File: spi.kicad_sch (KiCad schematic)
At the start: 15 parts, among them J3 Micro_SD_Card

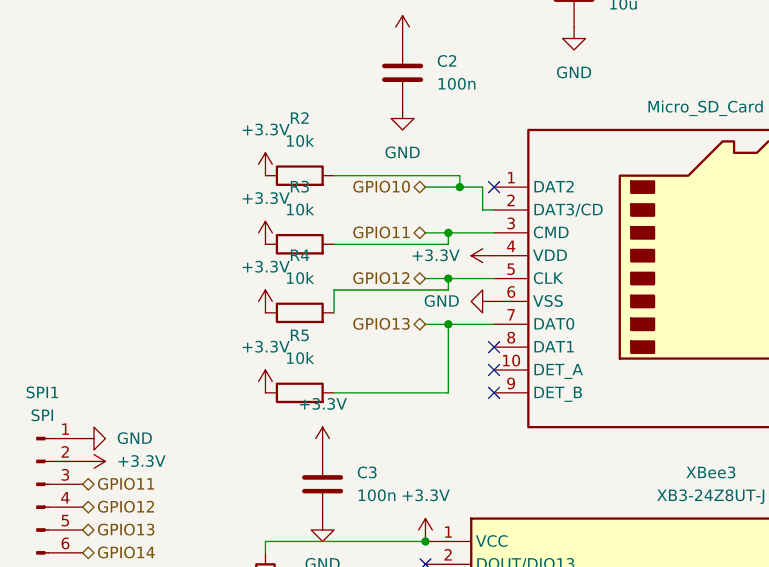
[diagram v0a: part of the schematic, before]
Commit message: Updated to v1.2 to address remaining issues
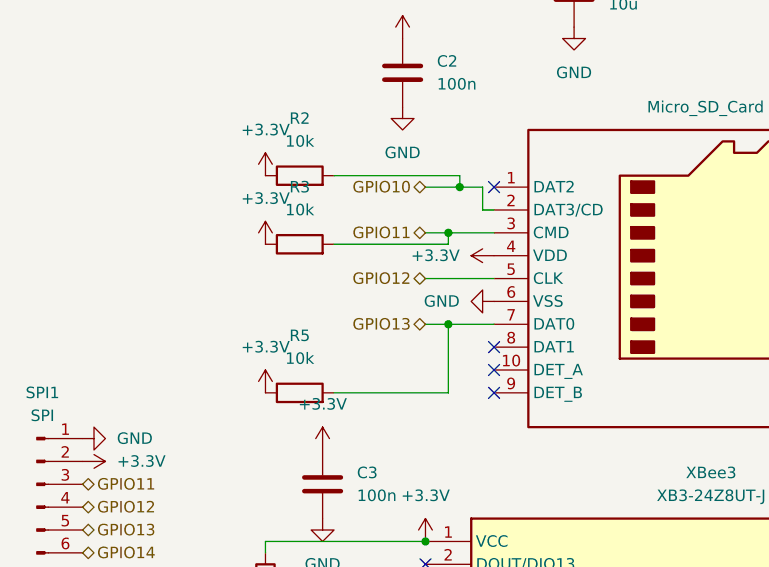
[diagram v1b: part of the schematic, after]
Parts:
- removed R4: 10k, Resistor_SMD:R_0603_1608Metric, symbol Device:R
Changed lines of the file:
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@@
 	)
 	(junction
-		(at 113.03 68.58)
-		(diameter 0)
-		(color 0 0 0 0)
-	)
-	(junction
 		(at 110.49 97.79)
 		(diameter 0)
@@
 	(wire
 		(pts
-			(xy 100.33 69.85) (xy 113.03 69.85)
-		)
-		(stroke
-			(width 0)
-			(type default)
-		)
-	)
-	(wire
-		(pts
 			(xy 113.03 81.28) (xy 113.03 73.66)
 		)
@@
 	(wire
 		(pts
-			(xy 100.33 72.39) (xy 100.33 69.85)
-		)
-		(stroke
-			(width 0)
-			(type default)
-		)
-	)
-	(wire
-		(pts
 			(xy 100.33 64.77) (xy 113.03 64.77)
 		)
@@
 	(wire
 		(pts
-			(xy 113.03 68.58) (xy 118.11 68.58)
+			(xy 110.49 68.58) (xy 118.11 68.58)
 		)
 		(stroke
@@
 	(wire
 		(pts
-			(xy 110.49 68.58) (xy 113.03 68.58)
-		)
-		(stroke
-			(width 0)
-			(type default)
-		)
-	)
-	(wire
-		(pts
-			(xy 113.03 68.58) (xy 113.03 69.85)
-		)
-		(stroke
-			(width 0)
-			(type default)
-		)
-	)
-	(wire
-		(pts
 			(xy 116.84 60.96) (xy 118.11 60.96)
 		)
@@
 	)
 	(symbol
-		(lib_id "Device:R")
-		(at 96.52 72.39 90)
-		(unit 1)
-		(exclude_from_sim no)
-		(in_bom yes)
-		(on_board yes)
-		(dnp no)
-		(fields_autoplaced yes)
-		(property "Reference" "R4"
-			(at 96.52 66.04 90)
-			(effects
-				(font
-					(size 1.27 1.27)
-				)
-			)
-		)
-		(property "Value" "10k"
-			(at 96.52 68.58 90)
-			(effects
-				(font
-					(size 1.27 1.27)
-				)
-			)
-		)
-		(property "Footprint" "Resistor_SMD:R_0603_1608Metric"
-			(at 96.52 74.168 90)
-			(effects
-				(font
-					(size 1.27 1.27)
-				)
-				(hide yes)
-			)
-		)
-		(property "Datasheet" "~"
-			(at 96.52 72.39 0)
-			(effects
-				(font
-					(size 1.27 1.27)
-				)
-				(hide yes)
-			)
-		)
-		(property "Description" "Resistor"
-			(at 96.52 72.39 0)
-			(effects
-				(font
-					(size 1.27 1.27)
-				)
-				(hide yes)
-			)
-		)
-		(pin "1"
-		)
-		(pin "2"
-		)
-		(instances
-			(project "AmidalaShield"
-				(path "/6d8d0000-f03d-4277-95db-0f566c3960c4/badd9ffd-b17a-400a-923e-2e73780848ba"
-					(reference "R4")
-					(unit 1)
-				)
-			)
-		)
-	)
-	(symbol
 		(lib_id "power:+3.3V")
 		(at 121.92 133.35 0)
@@
 					(unit 1)
 				)
-			)
-		)
-	)
-	(symbol
-		(lib_id "power:+3.3V")
-		(at 92.71 72.39 0)
-		(unit 1)
-		(exclude_from_sim no)
-		(in_bom yes)
-		(on_board yes)
-		(dnp no)
-		(fields_autoplaced yes)
-		(property "Reference" "#PWR023"
-			(at 92.71 76.2 0)
-			(effects
-				(font
-					(size 1.27 1.27)
-				)
-				(hide yes)
-			)
-		)
-		(property "Value" "+3.3V"
-			(at 92.71 67.31 0)
-			(effects
-				(font
-					(size 1.27 1.27)
-				)
-			)
-		)
-		(property "Footprint" ""
-			(at 92.71 72.39 0)
-			(effects
-				(font
-					(size 1.27 1.27)
-				)
-				(hide yes)
-			)
-		)
-		(property "Datasheet" ""
-			(at 92.71 72.39 0)
-			(effects
-				(font
-					(size 1.27 1.27)
-				)
-				(hide yes)
-			)
-		)
-		(property "Description" "Power symbol creates a global label with name \"+3.3V\""
-			(at 92.71 72.39 0)
-			(effects
-				(font
-					(size 1.27 1.27)
-				)
-				(hide yes)
-			)
-		)
-		(pin "1"
-		)
-		(instances
-			(project "AmidalaShield"
-				(path "/6d8d0000-f03d-4277-95db-0f566c3960c4/badd9ffd-b17a-400a-923e-2e73780848ba"
-					(reference "#PWR023")
-					(unit 1)
-				)
